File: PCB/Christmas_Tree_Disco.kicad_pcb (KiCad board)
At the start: 2 copper layers, 190.5 x 188.9 mm, 35 parts, among them U1 DEV_KIT_EK-TM4C123GXL, U2 TLC5955DCA

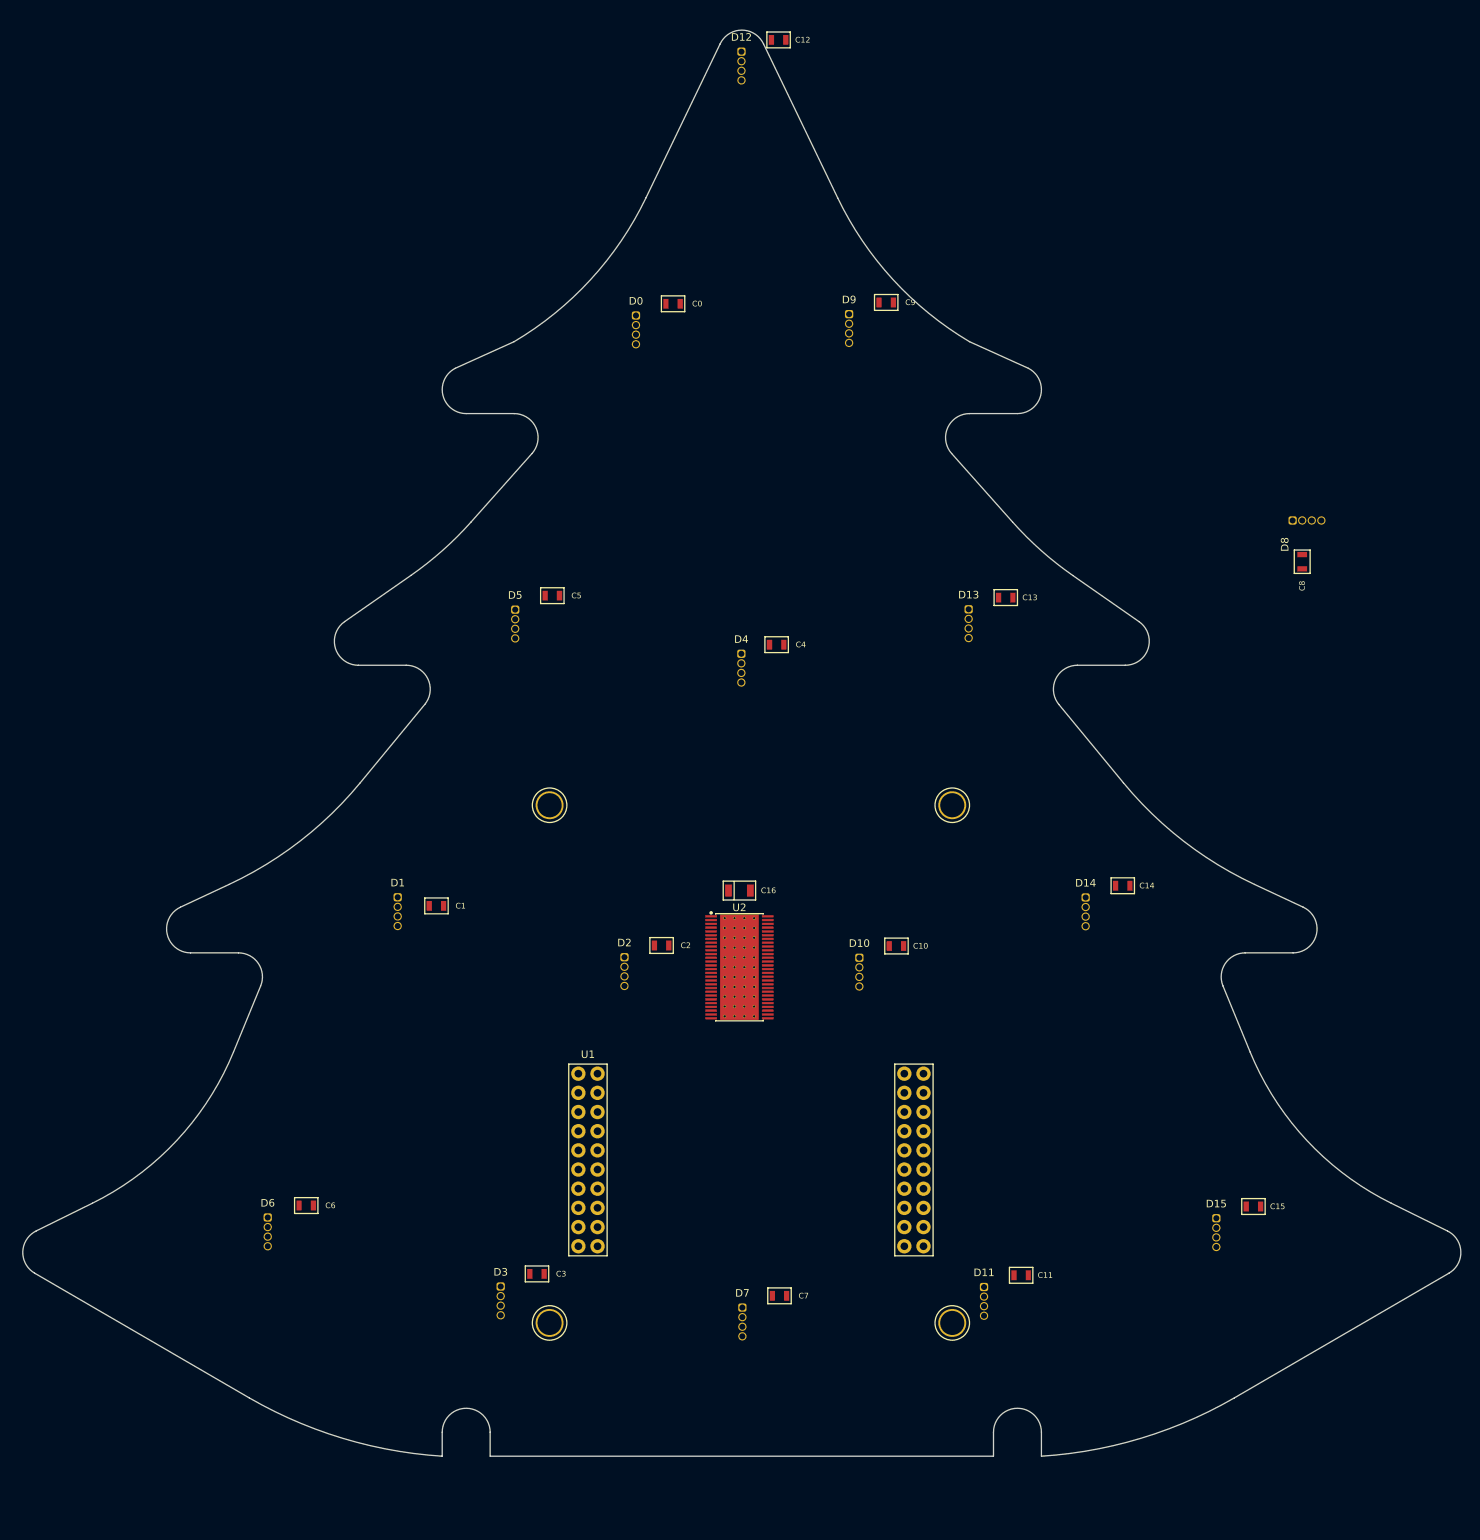
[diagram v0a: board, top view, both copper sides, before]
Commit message: Preliminary PCB layout
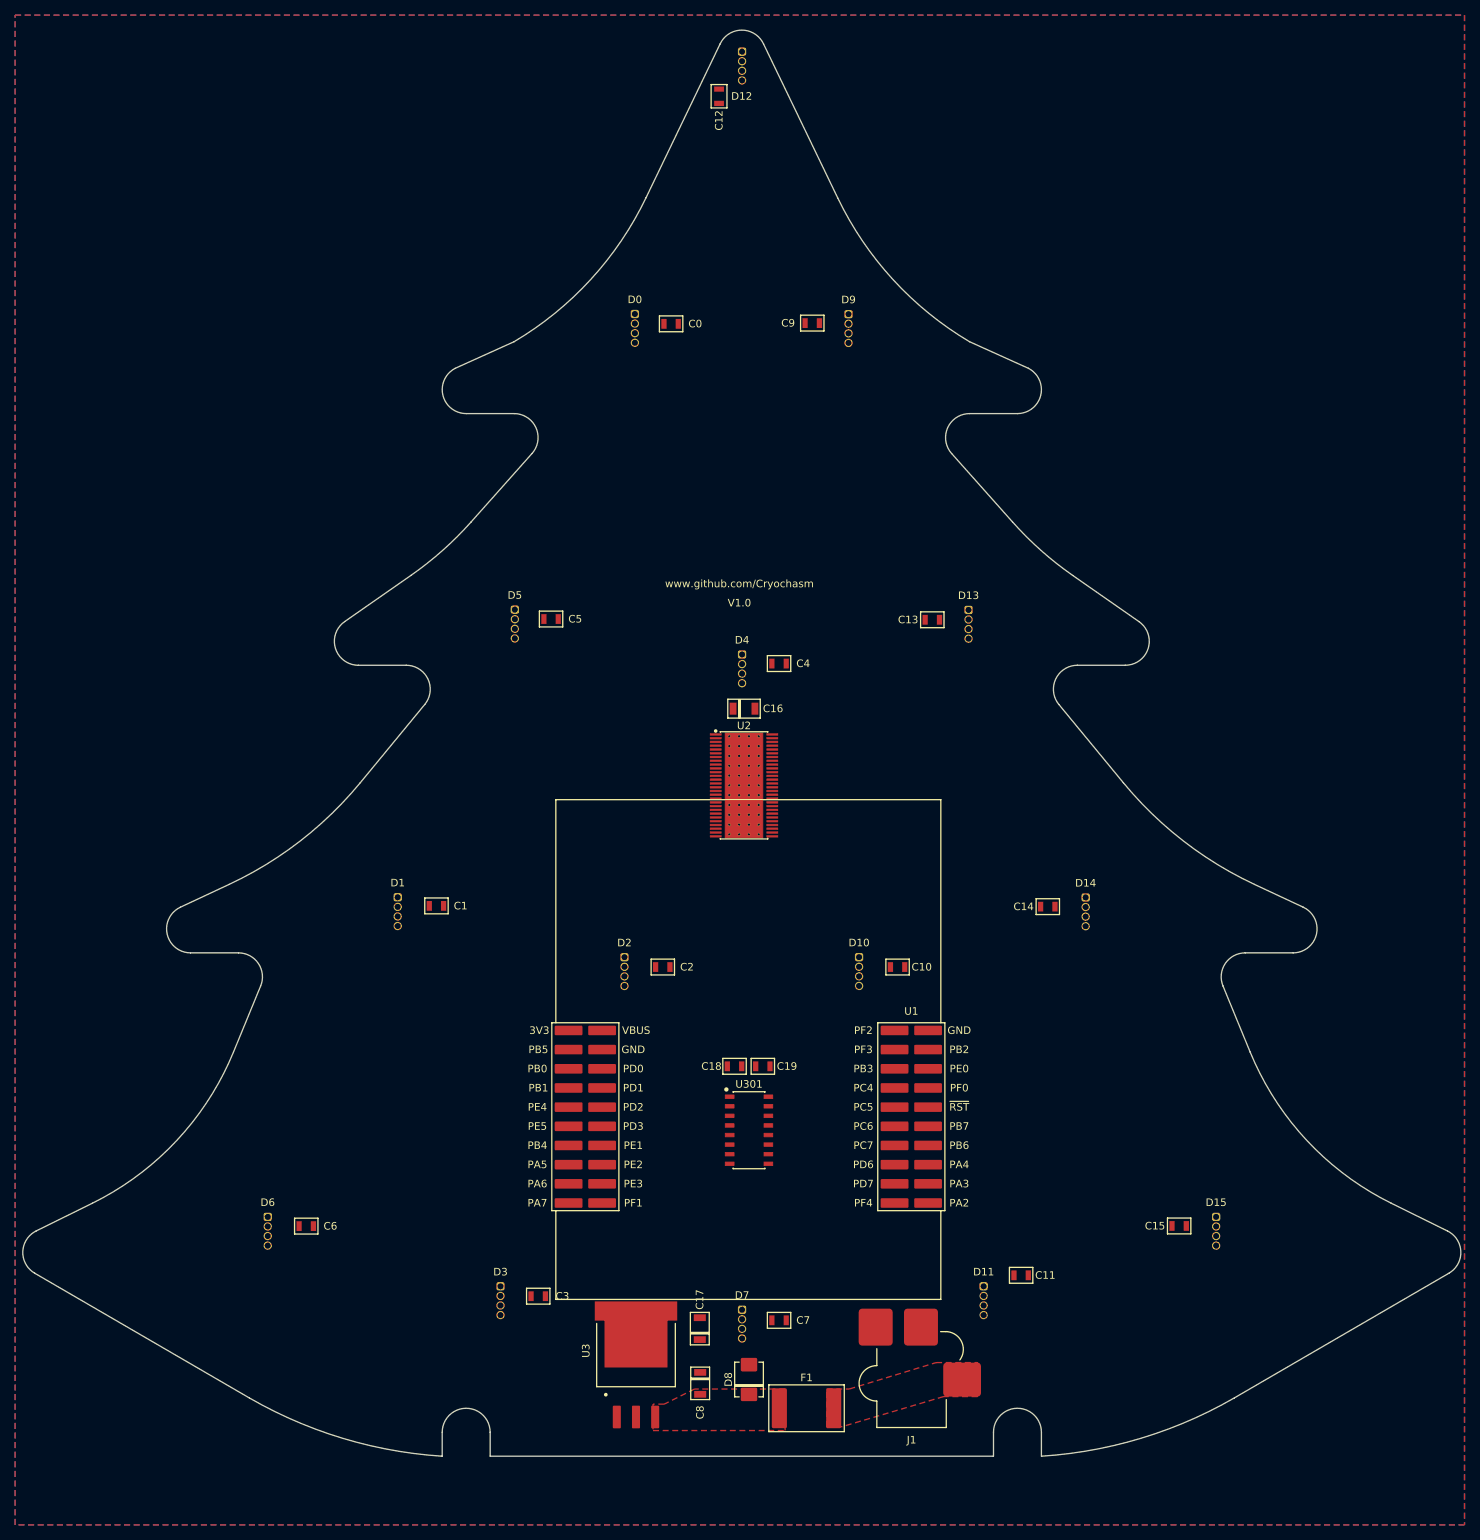
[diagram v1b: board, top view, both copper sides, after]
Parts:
- added C17: Capacitor-Pol, local:SMD-POL-1206, F.Cu at (102.7, 199.0)
- added C18: Capacitor, local:SMD-0805, F.Cu at (107.3, 164.2)
- added C19: Capacitor, local:SMD-0805, F.Cu at (111.0, 164.2)
- added F1: 24V 3A, local:SMD-2920, F.Cu at (116.8, 209.6)
- added H3: Snow Silk Screen, local:snow, B.Cu at (108.6, 124.0)
- added H301: 2x10 HEADER, local:2x10_header_3d, F.Cu at (87.5, 171.0)
- added H302: 2x10 HEADER, local:2x10_header_3d, F.Cu at (130.8, 171.0)
- added J1: PJ-006B-SMT-TR, local:PJ-006B-SMT, F.Cu at (130.8, 205.8)
- added U3: LM1085-5.0, local:TO-263, F.Cu at (94.2, 202.2)
- added U301: MC14504B, local:SOIC-16, F.Cu at (109.2, 172.7)
- added V1.0: www.github.com/Cryochasm, local:PCB-LABEL, F.Cu at (108.0, 101.6)
- C8: value Capacitor -> Capacitor-Pol; footprint local:SMD-0805 -> local:SMD-POL-1206
- D8: value RGB LED -> TVS-Bidirectional; footprint local:T-1_5mm -> local:DO-214AA
- moved D8 135.7 mm to (109.2, 205.7)
- moved C8 134.9 mm to (102.8, 206.2)
- moved C16 24.1 mm to (108.6, 116.9)
- moved U2 24.1 mm to (108.6, 127.0)
- moved U1 23.2 mm to (109.1, 170.9)
- moved C12 10.9 mm to (105.2, 35.8), turned to 270 degrees
- moved C14 10.3 mm to (148.8, 143.1), turned to 180 degrees
- moved C15 10.2 mm to (166.2, 185.4), turned to 180 degrees
- moved C9 10.2 mm to (117.6, 65.8), turned to 180 degrees
- moved C13 10.2 mm to (133.5, 105.1), turned to 180 degrees
- moved C7 3.24 mm to (113.2, 197.9)
- moved C5 3.10 mm to (83.0, 105.0)
- moved C3 2.95 mm to (81.3, 194.7)
- moved C2 2.86 mm to (97.8, 151.1)
- moved C10 2.79 mm to (128.9, 151.1)
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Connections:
- C0 pad 1: /Top Sheet/RGB LED Array/5V -> /Top Sheet/Microcontroller/5V
- C0 pad 2: /Top Sheet/RGB LED Array/GND -> /Top Sheet/Microcontroller/GND
- C1 pad 1: /Top Sheet/RGB LED Array/5V -> /Top Sheet/Microcontroller/5V
- C1 pad 2: /Top Sheet/RGB LED Array/GND -> /Top Sheet/Microcontroller/GND
- C10 pad 1: /Top Sheet/RGB LED Array/5V -> /Top Sheet/Microcontroller/5V
- C10 pad 2: /Top Sheet/RGB LED Array/GND -> /Top Sheet/Microcontroller/GND
- C11 pad 1: /Top Sheet/RGB LED Array/5V -> /Top Sheet/Microcontroller/5V
- C11 pad 2: /Top Sheet/RGB LED Array/GND -> /Top Sheet/Microcontroller/GND
- C12 pad 1: /Top Sheet/RGB LED Array/5V -> /Top Sheet/Microcontroller/5V
- C12 pad 2: /Top Sheet/RGB LED Array/GND -> /Top Sheet/Microcontroller/GND
- C13 pad 1: /Top Sheet/RGB LED Array/5V -> /Top Sheet/Microcontroller/5V
- C13 pad 2: /Top Sheet/RGB LED Array/GND -> /Top Sheet/Microcontroller/GND
- C14 pad 1: /Top Sheet/RGB LED Array/5V -> /Top Sheet/Microcontroller/5V
- C14 pad 2: /Top Sheet/RGB LED Array/GND -> /Top Sheet/Microcontroller/GND
- C15 pad 1: /Top Sheet/RGB LED Array/5V -> /Top Sheet/Microcontroller/5V
- C15 pad 2: /Top Sheet/RGB LED Array/GND -> /Top Sheet/Microcontroller/GND
- C16 pad 1: /Top Sheet/RGB LED Array/GND -> /Top Sheet/Microcontroller/GND
- C16 pad 2: /Top Sheet/RGB LED Array/5V -> /Top Sheet/Microcontroller/5V
- C2 pad 1: /Top Sheet/RGB LED Array/5V -> /Top Sheet/Microcontroller/5V
- C2 pad 2: /Top Sheet/RGB LED Array/GND -> /Top Sheet/Microcontroller/GND
- C3 pad 1: /Top Sheet/RGB LED Array/5V -> /Top Sheet/Microcontroller/5V
- C3 pad 2: /Top Sheet/RGB LED Array/GND -> /Top Sheet/Microcontroller/GND
- C4 pad 1: /Top Sheet/RGB LED Array/5V -> /Top Sheet/Microcontroller/5V
- C4 pad 2: /Top Sheet/RGB LED Array/GND -> /Top Sheet/Microcontroller/GND
- C5 pad 1: /Top Sheet/RGB LED Array/5V -> /Top Sheet/Microcontroller/5V
- C5 pad 2: /Top Sheet/RGB LED Array/GND -> /Top Sheet/Microcontroller/GND
- C6 pad 1: /Top Sheet/RGB LED Array/5V -> /Top Sheet/Microcontroller/5V
- C6 pad 2: /Top Sheet/RGB LED Array/GND -> /Top Sheet/Microcontroller/GND
- C7 pad 1: /Top Sheet/RGB LED Array/5V -> /Top Sheet/Microcontroller/5V
- C7 pad 2: /Top Sheet/RGB LED Array/GND -> /Top Sheet/Microcontroller/GND
- C8 pad 1: /Top Sheet/RGB LED Array/5V -> /Top Sheet/Microcontroller/GND
- C8 pad 2: /Top Sheet/RGB LED Array/GND -> Net-(C8-Pad2)
- C9 pad 1: /Top Sheet/RGB LED Array/5V -> /Top Sheet/Microcontroller/5V
- C9 pad 2: /Top Sheet/RGB LED Array/GND -> /Top Sheet/Microcontroller/GND
- D0 pad 2: /Top Sheet/RGB LED Array/5V -> /Top Sheet/Microcontroller/5V
- D1 pad 2: /Top Sheet/RGB LED Array/5V -> /Top Sheet/Microcontroller/5V
- D10 pad 2: /Top Sheet/RGB LED Array/5V -> /Top Sheet/Microcontroller/5V
- D11 pad 2: /Top Sheet/RGB LED Array/5V -> /Top Sheet/Microcontroller/5V
- D12 pad 2: /Top Sheet/RGB LED Array/5V -> /Top Sheet/Microcontroller/5V
- D13 pad 2: /Top Sheet/RGB LED Array/5V -> /Top Sheet/Microcontroller/5V
- D14 pad 2: /Top Sheet/RGB LED Array/5V -> /Top Sheet/Microcontroller/5V
- D15 pad 2: /Top Sheet/RGB LED Array/5V -> /Top Sheet/Microcontroller/5V
- D2 pad 2: /Top Sheet/RGB LED Array/5V -> /Top Sheet/Microcontroller/5V
- D3 pad 2: /Top Sheet/RGB LED Array/5V -> /Top Sheet/Microcontroller/5V
- D4 pad 2: /Top Sheet/RGB LED Array/5V -> /Top Sheet/Microcontroller/5V
- D5 pad 2: /Top Sheet/RGB LED Array/5V -> /Top Sheet/Microcontroller/5V
- D6 pad 2: /Top Sheet/RGB LED Array/5V -> /Top Sheet/Microcontroller/5V
- D7 pad 2: /Top Sheet/RGB LED Array/5V -> /Top Sheet/Microcontroller/5V
- D8 pad 1: /Top Sheet/RGB LED Array/RGB08_1 -> Net-(C8-Pad2)
- D8 pad 2: /Top Sheet/RGB LED Array/5V -> /Top Sheet/Microcontroller/GND
- D9 pad 2: /Top Sheet/RGB LED Array/5V -> /Top Sheet/Microcontroller/5V
- U1 pad 1: Net-(U1-Pad1) -> /Top Sheet/Microcontroller/3V3
- U2 pad 1: /Top Sheet/RGB LED Array/DATA -> /Top Sheet/Microcontroller/DATA
- U2 pad 2: /Top Sheet/RGB LED Array/SCLK -> /Top Sheet/Microcontroller/SCLK
- U2 pad 28: /Top Sheet/RGB LED Array/ERROR_RD -> /Top Sheet/Microcontroller/ERROR_RD
- U2 pad 29: /Top Sheet/RGB LED Array/GND -> /Top Sheet/Microcontroller/GND
- U2 pad 3: /Top Sheet/RGB LED Array/LAT -> /Top Sheet/Microcontroller/LAT
- U2 pad 51: /Top Sheet/RGB LED Array/RGB08_2 -> Net-(U2-Pad51)
- U2 pad 52: /Top Sheet/RGB LED Array/RGB08_1 -> Net-(U2-Pad52)
- U2 pad 53: /Top Sheet/RGB LED Array/RGB08_0 -> Net-(U2-Pad53)
- U2 pad 54: /Top Sheet/RGB LED Array/5V -> /Top Sheet/Microcontroller/5V
- U2 pad 55: /Top Sheet/RGB LED Array/GSCLK -> /Top Sheet/Microcontroller/GSCLK
- U2 pad 56: /Top Sheet/RGB LED Array/GND -> /Top Sheet/Microcontroller/GND
- U2 pad EP: /Top Sheet/RGB LED Array/GND -> /Top Sheet/Microcontroller/GND
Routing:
- added copper zone on B.Cu, net /Top Sheet/Microcontroller/GND
- added copper zone on F.Cu, net /Top Sheet/Microcontroller/GND
- added copper zone on F.Cu, net /Top Sheet/Power Supply/VIN
- added copper zone on F.Cu, net Net-(C8-Pad2)
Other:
- net class Default: clearance 0 -> 0.15; via_dia 0.8 -> 0.686; via_drill 0.4 -> 0.432
- rule trace_clearance: 0 -> 0.15
- board text removed: "12.5000"
